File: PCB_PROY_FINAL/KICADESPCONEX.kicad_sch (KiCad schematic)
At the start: 36 parts, among them IC1 USBLC6-2SC6, IC2 ESP32-S3-WROOM-1-N16, J1 Connector, USB-TYPE-C-16P

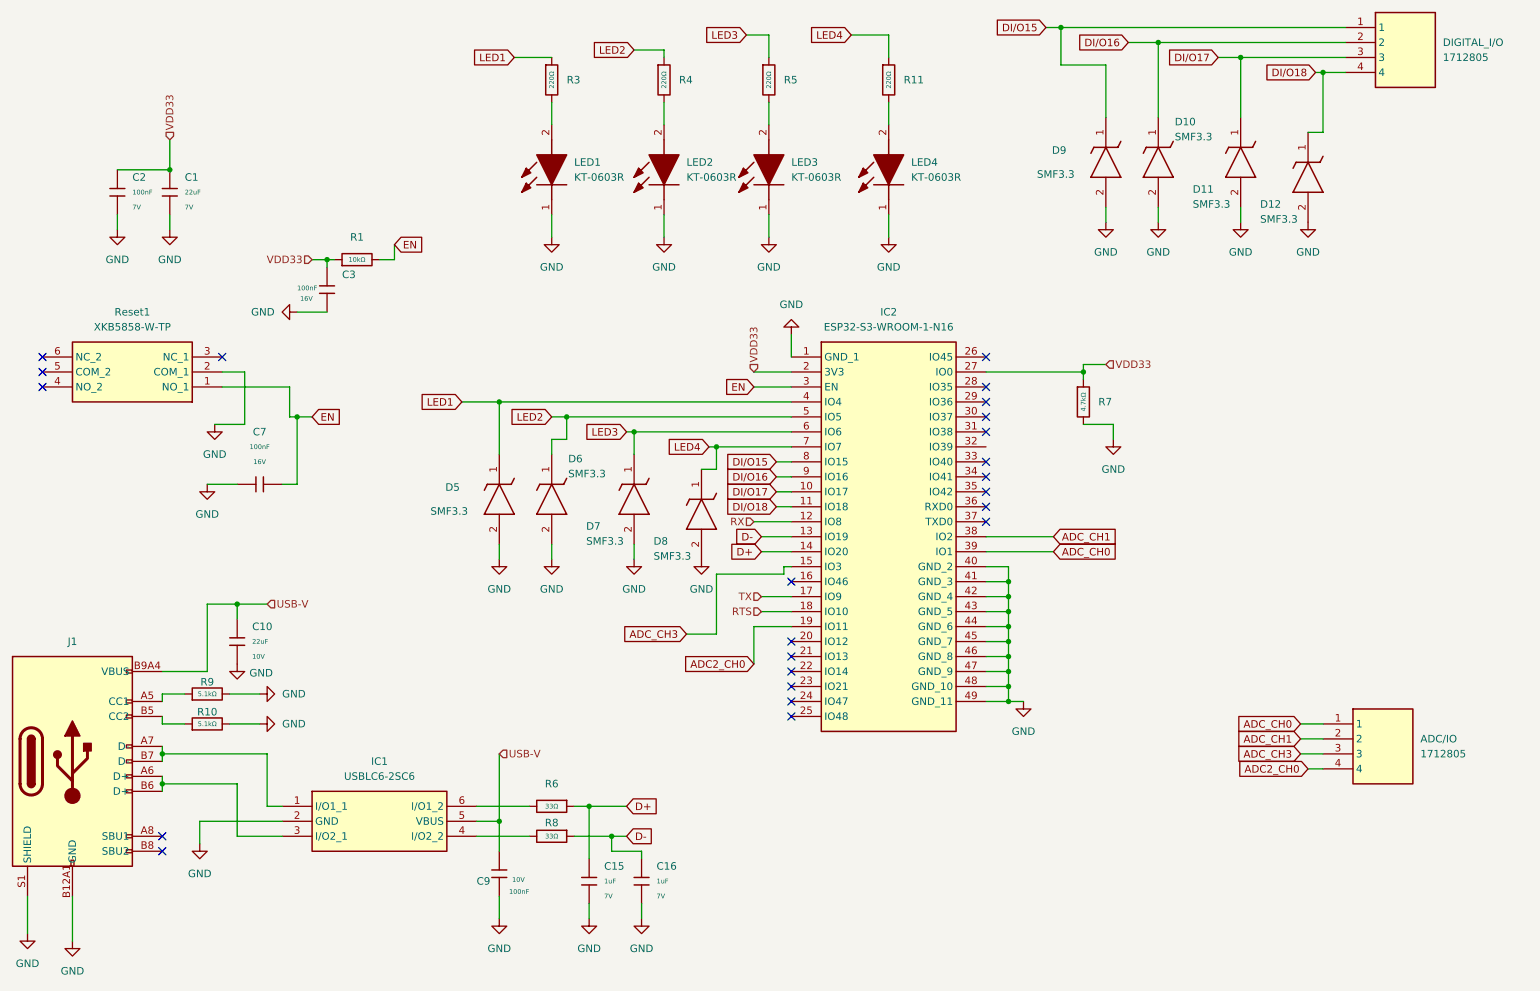
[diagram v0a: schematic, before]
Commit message: Last update pcb
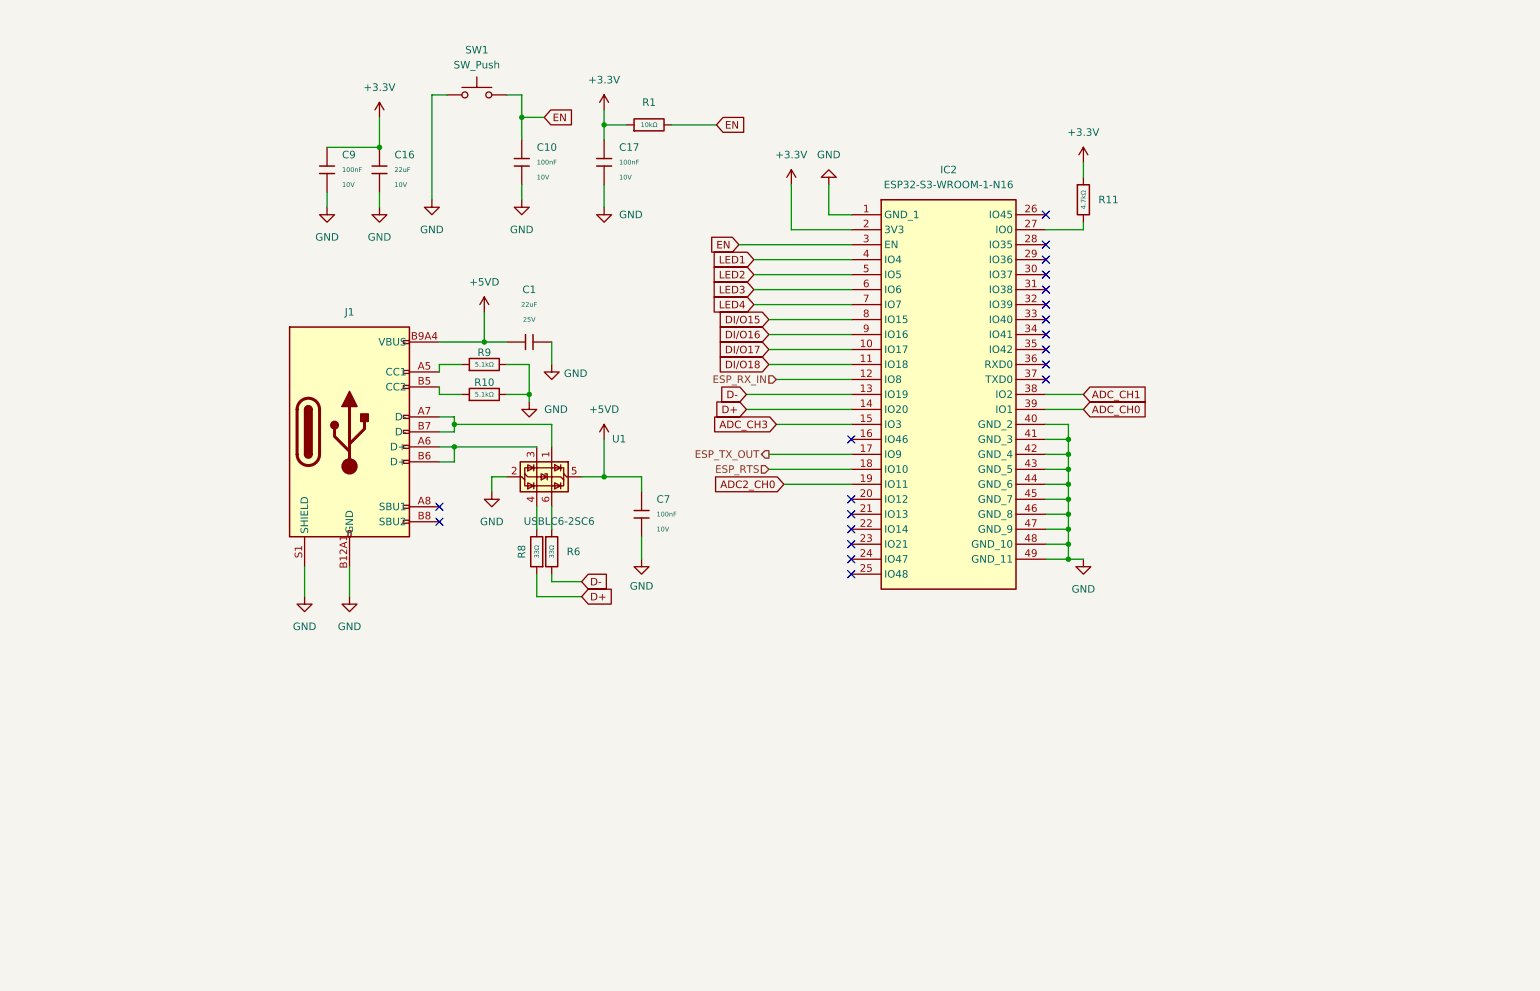
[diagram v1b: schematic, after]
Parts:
- removed ADC/IO, DIGITAL_I/O: 1712805, SamacSys_Parts:1712805, symbol SamacSys_Parts:1712805
- removed C1, C10: 22uF, PCM_JLCPCB:C_0603, symbol PCM_JLCPCB-Capacitors:0603,22uF
- removed C15, C16: 1uF, PCM_JLCPCB:C_0402, symbol PCM_JLCPCB-Capacitors:0402,1uF
- removed C2, C3, C7, C9: 100nF, PCM_JLCPCB:C_0402, symbol PCM_JLCPCB-Capacitors:0402,100nF
- removed D10, D11, D12, D5, D6, D7, D8, D9: SMF3.3, SamacSys_Parts:SOD3718X108N, symbol SamacSys_Parts:SMF3.3
- removed IC1: USBLC6-2SC6, SamacSys_Parts:SOT95P280X145-6N, symbol SamacSys_Parts:USBLC6-2SC6
- removed LED1, LED2, LED3, LED4: KT-0603R, LEDC1608X70N, symbol SamacSys_Parts:KT-0603R
- removed R11, R3, R4, R5: 220Ω, PCM_JLCPCB:R_0402, symbol PCM_JLCPCB-Resistors:0402,220Ω
- removed R7: 4.7kΩ, PCM_JLCPCB:R_0402, symbol PCM_JLCPCB-Resistors:0402,4.7kΩ
- removed Reset1: XKB5858-W-TP, SamacSys_Parts:XKB5858WTP, symbol SamacSys_Parts:XKB5858-W-TP
- added C1: 22uF, PCM_JLCPCB:C_0805, symbol PCM_JLCPCB-Capacitors:0805,22uF
- added C10, C17, C7, C9: 100nF, PCM_JLCPCB:C_0603, symbol PCM_JLCPCB-Capacitors:0603,100nF
- added C16: 22uF, PCM_JLCPCB:C_1206, symbol PCM_JLCPCB-Capacitors:1206,22uF
- added R11: 4.7kΩ, PCM_JLCPCB:R_1206, symbol PCM_JLCPCB-Resistors:1206,4.7kΩ
- added SW1: SW_Push, SamacSys_Parts:XKB5858WTP, symbol Switch:SW_Push
- added U1: USBLC6-2SC6, Package_TO_SOT_SMD:SOT-23-6, symbol Power_Protection:USBLC6-2SC6
- IC2: LCSC (none) -> C2913199
- R1: LCSC C25744 -> C4139000
- R6, R8: LCSC C25105 -> C2122351
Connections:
- net D+: now also R8.1; no longer R6.1
- net D-: now also R6.2; no longer R8.1
- net EN: now also C10.1, SW1.2
- net GND: now also C1.2, C10.2, C16.2, C17.2, C7.2, C9.2, SW1.1, U1.2 (GND)
- net at J1.A7 (D-), J1.B7 (D-): now also U1.1 (I/O1)
- net at J1.A6 (D+), J1.B6 (D+): now also U1.3 (I/O2)
- net at R8.2: now also U1.4 (I/O2)
- net RTS renamed ESP_RTS
- net RX renamed ESP_RX_IN
- net TX renamed ESP_TX_OUT
- net USB-V renamed +5VD
- net +5VD: now also C1.1, C7.1, U1.5 (VBUS)
- net VDD33 renamed +3.3V
- net +3.3V: now also C16.1, C17.1, C9.1, R11.1; no longer IC2.27 (IO0)
- new net: R6.1, U1.6 (I/O1)
- new net: IC2.27 (IO0), R11.2
- no-connect marks 23 -> 20
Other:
- moved on the sheet: IC2, J1, R1, R10, R6, R8, R9
